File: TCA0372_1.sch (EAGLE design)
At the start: 30 parts, among them IC1R1 AQY212_1, IC2 Dil16: 4xAQY212, IC4 TCA0372, Q1 BSS101, Q2 BSS101

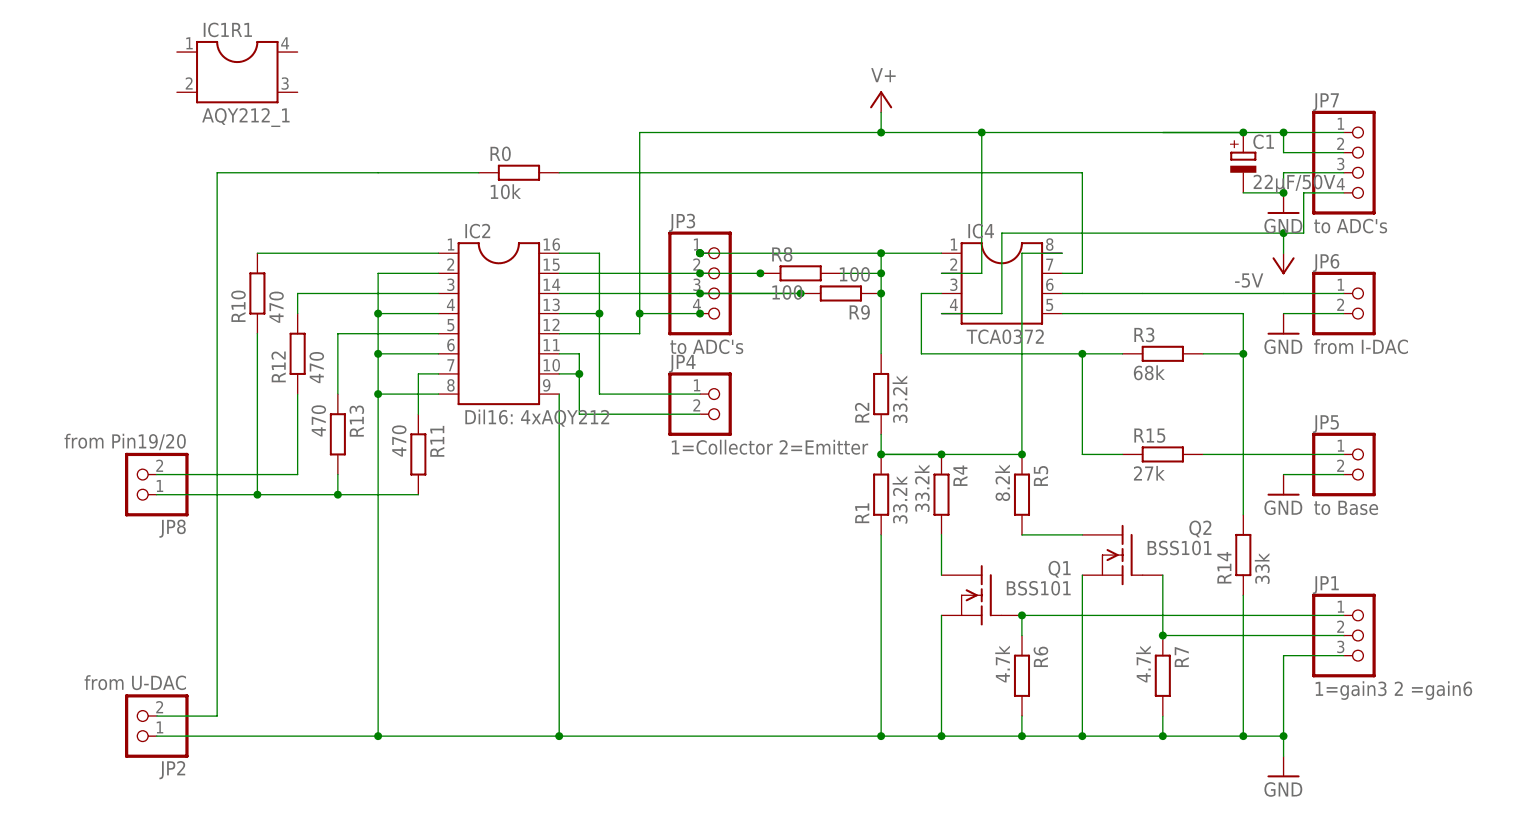
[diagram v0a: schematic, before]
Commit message: Add files via upload
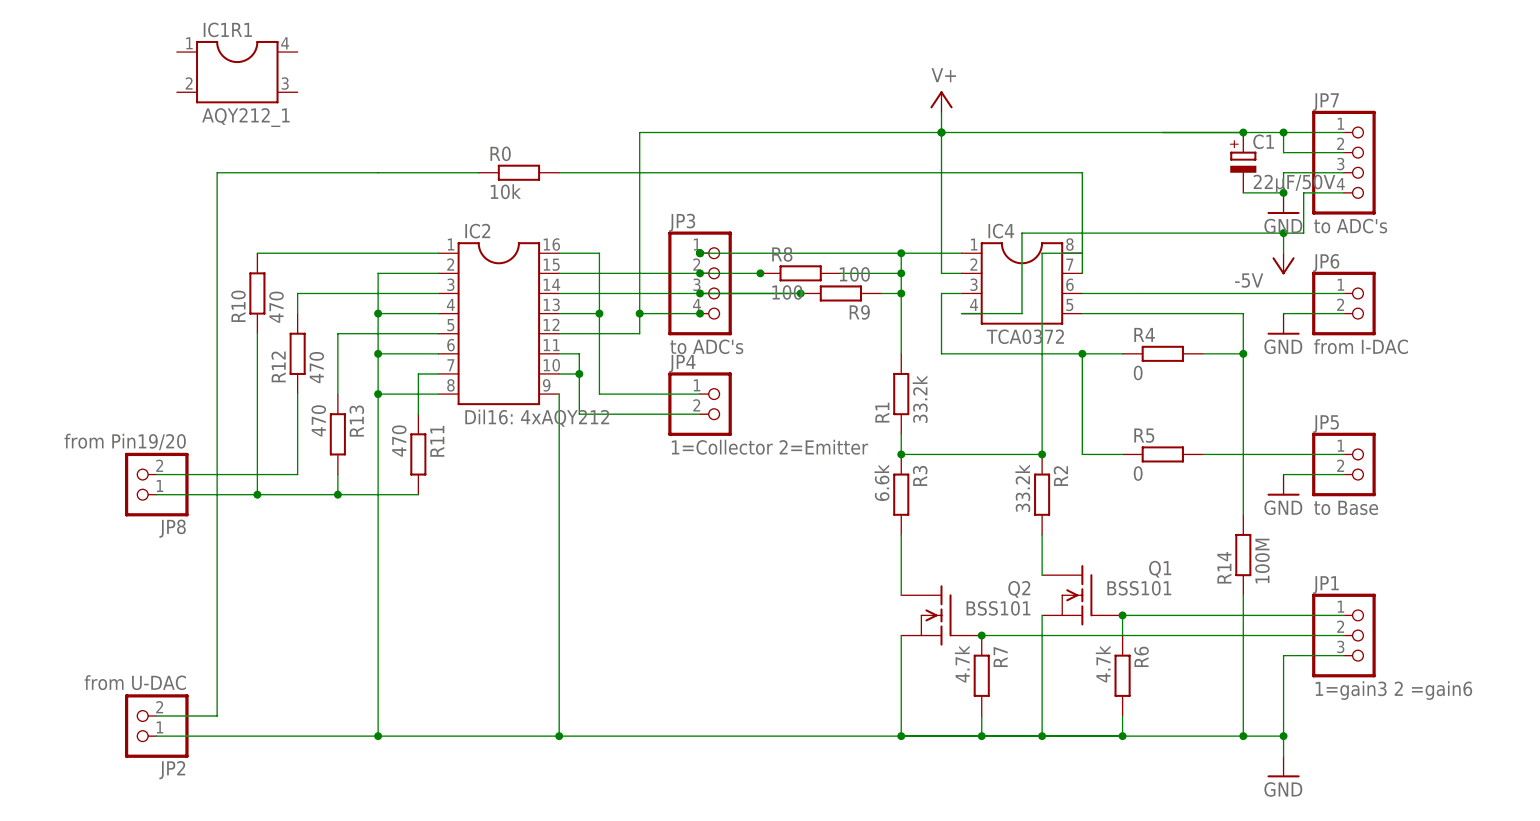
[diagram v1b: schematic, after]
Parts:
- removed R15: 27k, rcl:R-EU_0207/7
- R14: value 33k -> 100M
- R3: value 68k -> 6.6k
- R4: value 33.2k -> 0
- R5: value 8.2k -> 0
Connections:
- removed net N$14: IC4.1, JP3.1, R2.2, R8.2, R9.1
- removed net N$4: IC4.8, R1.2, R2.1, R4.1, R5.1
- new net N$21: IC4.1, JP3.1, R1.2, R8.2, R9.1
- new net N$22: IC4.8, R1.1, R2.1, R3.1
- net GND: no longer R1.1
- net N$1: now also R4.2; no longer R3.2
- net N$13: now also R4.1, R5.1; no longer R15.1, R3.1
- net N$20: now also R5.2; no longer R15.2
- net N$5: now also R2.2; no longer R4.2
- net N$6: now also R3.2; no longer R5.2
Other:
- moved on the sheet: IC4, Q1, Q2, R1, R2, R3, R4, R5, R6, R7
